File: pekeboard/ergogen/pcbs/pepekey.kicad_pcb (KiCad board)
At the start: 2 copper layers, 150.9 x 124.7 mm, 63 parts

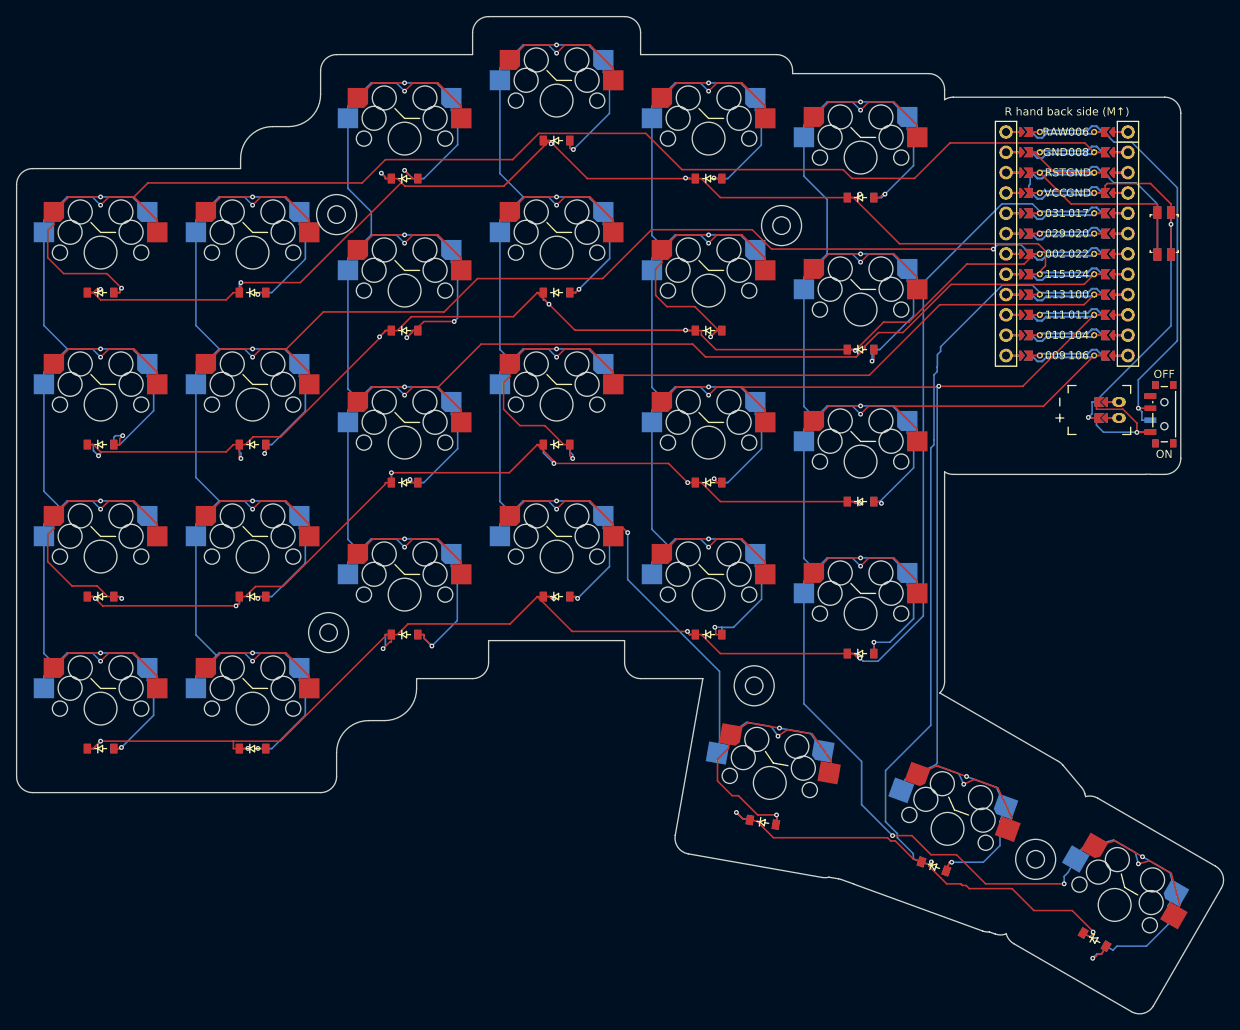
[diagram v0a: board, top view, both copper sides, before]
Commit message: pekepad folder fix
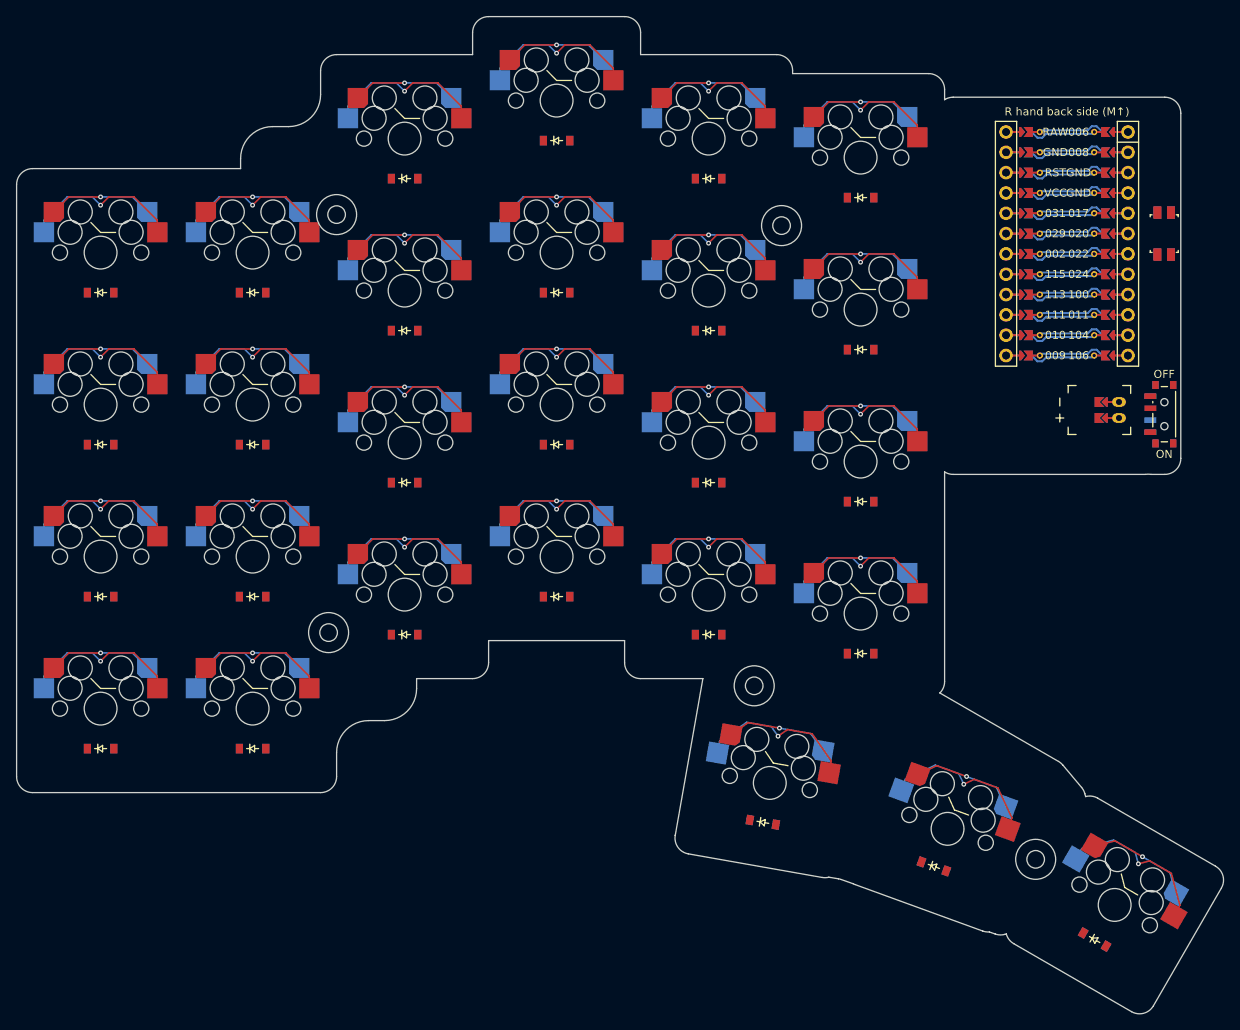
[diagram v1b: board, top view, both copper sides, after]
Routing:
- net (no net): track 0.00 -> 337.7 mm
- net P008: track 268.6 -> 42.3 mm
- net P031: track 206.8 -> 0.00 mm, vias 6 -> 0
- net P100: track 258.8 -> 52.9 mm, vias 6 -> 5
- net P011: track 258.2 -> 52.9 mm, vias 6 -> 5
- net P106: track 251.5 -> 52.9 mm, vias 7 -> 5
- net P022: track 240.4 -> 42.3 mm, vias 5 -> 4
- net P024: track 230.4 -> 42.3 mm
- net P115: track 164.6 -> 0.00 mm, vias 6 -> 0
- net P002: track 158.9 -> 0.00 mm, vias 6 -> 0
- net P113: track 154.5 -> 0.00 mm, vias 3 -> 0
- net P025: track 120.0 -> 0.00 mm, vias 6 -> 0
- net GND: track 89.7 -> 0.00 mm, vias 2 -> 0
- net RAW: track 56.1 -> 0.00 mm, vias 1 -> 0
- net RST: track 47.5 -> 0.00 mm
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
